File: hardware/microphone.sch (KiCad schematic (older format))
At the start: 9 parts, among them U3 MEMS-SPM0408LE5H, U4 OPA344

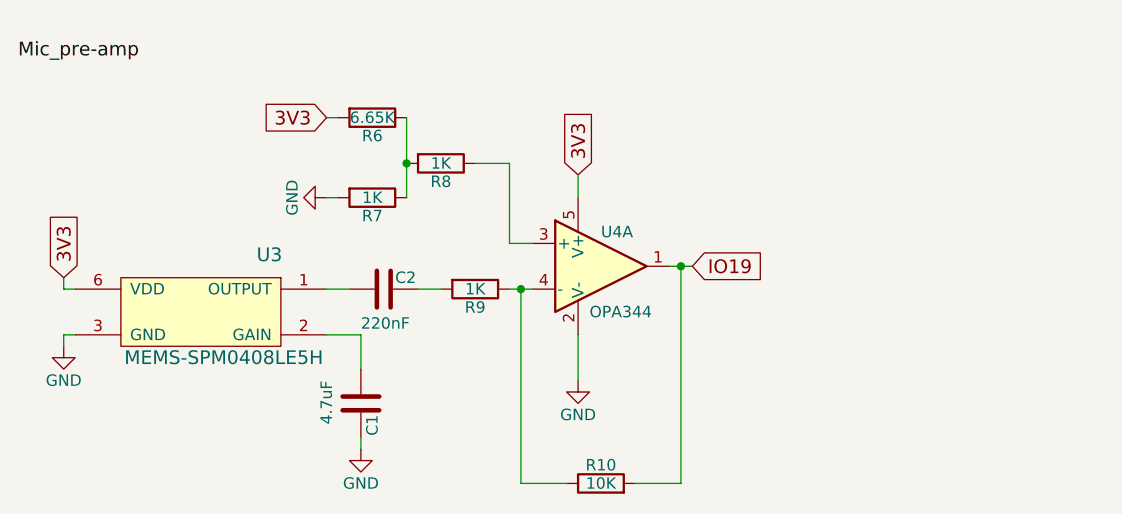
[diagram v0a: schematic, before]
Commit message: updatE
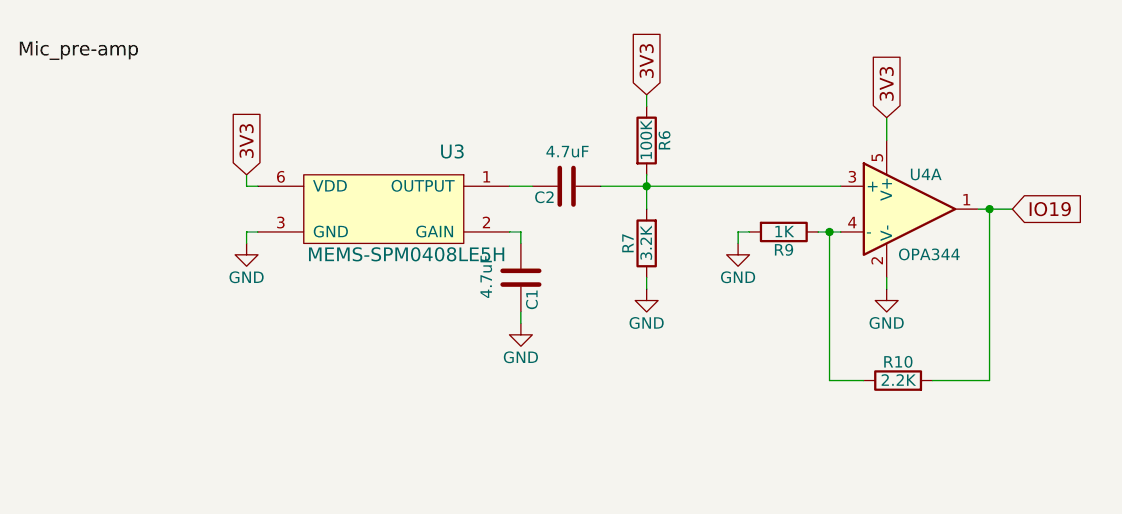
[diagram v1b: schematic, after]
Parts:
- removed R8: 1K, Resistors_SMD:R_0603_HandSoldering, symbol R
- C2: value 220nF -> 4.7uF; Part Number C1608X7R1C224K080AC -> CL10B475KQ8NQNC
- R10: value 10K -> 2.2K
- R6: value 6.65K -> 100K; Part Number RC0603FR-076K65L -> RC0603JR-07100KL
- R7: value 1K -> 3.2K; Part Number RC0603JR-071KL -> RC0402FR-073K24L
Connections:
- net 3V3: now also R6.1; no longer R6.2
- net GND: now also R7.1, R9.2; no longer R7.2
- net at U4.3 (+): now also C2.2, R6.2, R7.2
- net at C2.1: now also U3.1 (OUTPUT); no longer R9.2
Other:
- moved on the sheet: C1, R10, R9, U3, U4A
